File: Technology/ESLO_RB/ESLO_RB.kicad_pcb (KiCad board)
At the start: 4 copper layers, 50.5 x 20 mm, 80 parts, among them CN3 1000pF, CN4 1uF, CN7 1000pF, CN8 1uF, CN9 4700pF, J1 Board to Board, J2 Conn_01x10_Female, U1 TPS62740, U10 MT29F2G01ABBGDWB-IT:G TR, U2 LP5907MFX-1.5, U3 CC2652RB, U4 2450BM14G0011, U5 MAX1720, U6 TPS72301DDCT, U7 ADS1294, U8 LSM303AGR, U9 CY15V104QI-20LPXC

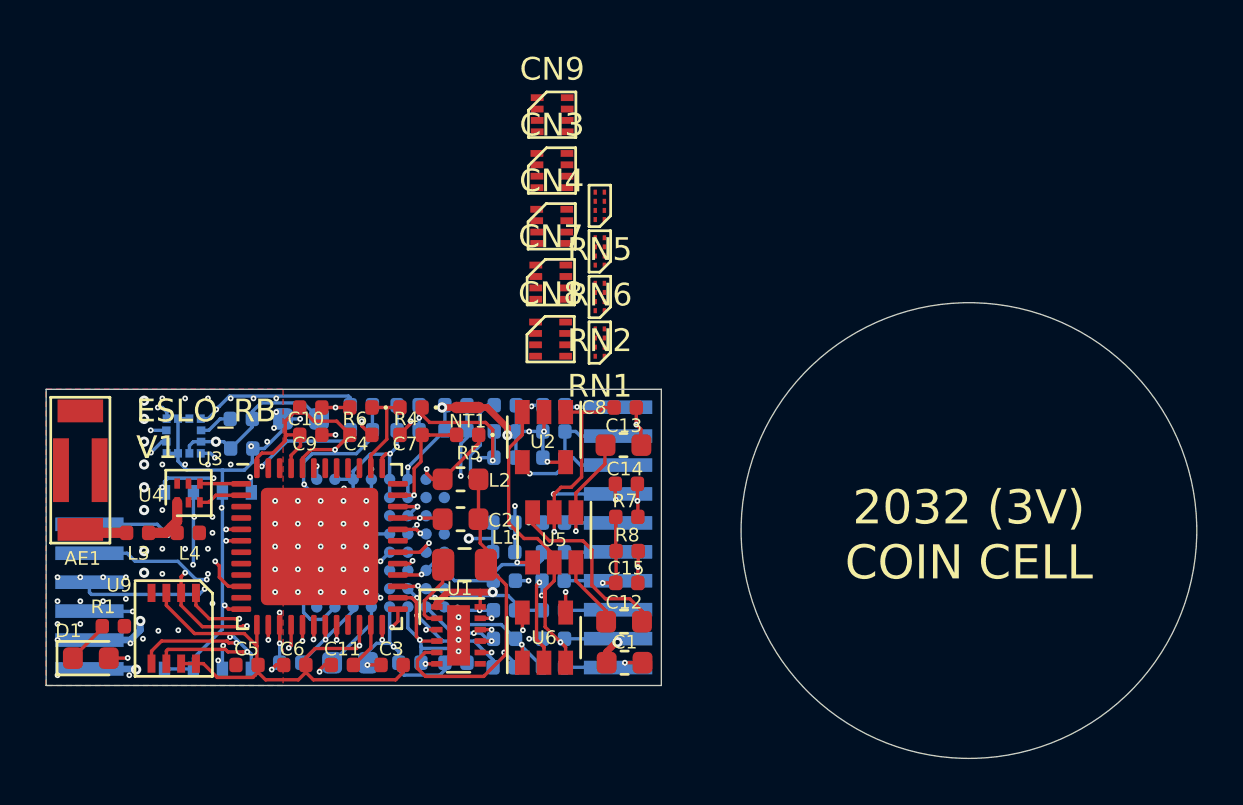
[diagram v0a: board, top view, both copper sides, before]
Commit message: Completed RB design
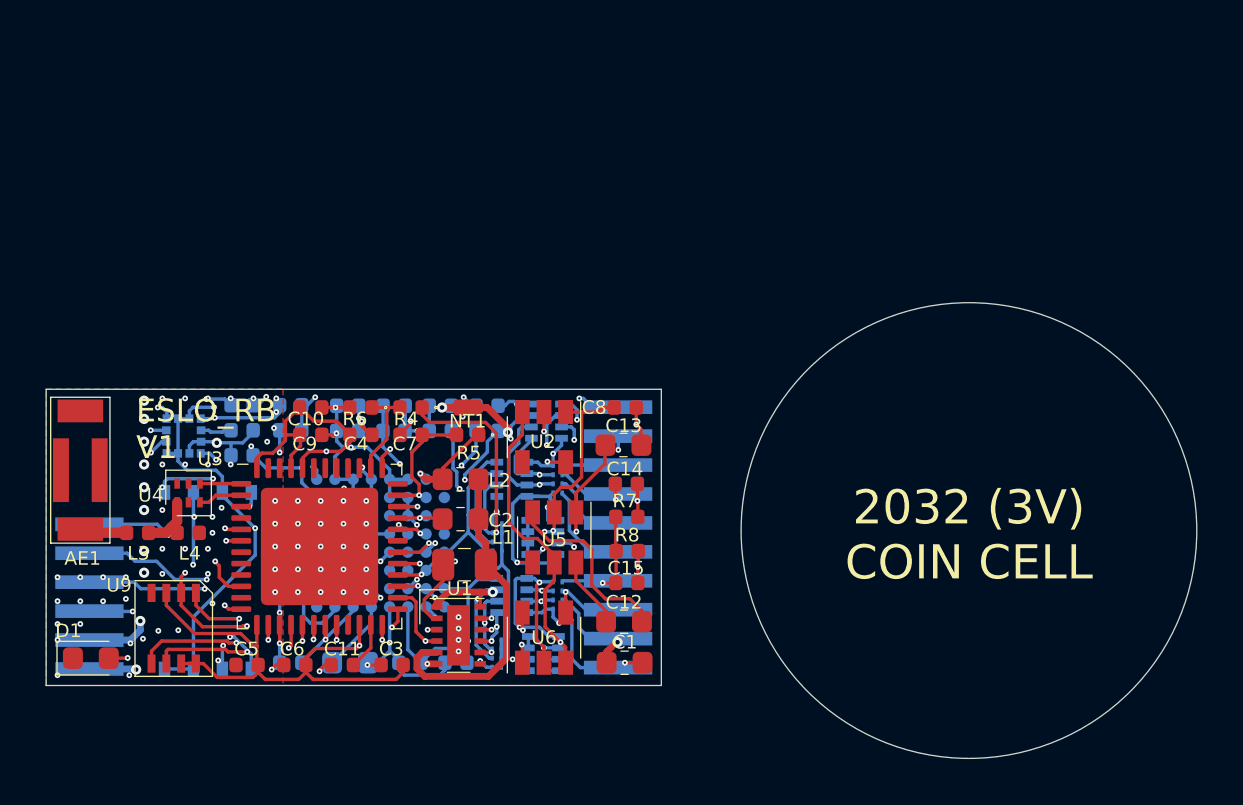
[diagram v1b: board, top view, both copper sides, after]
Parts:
- removed C18, C28: 1uF, Capacitor_SMD:C_0402_1005Metric
- removed C22, C24, C25: 4.7nF, Capacitor_SMD:C_0402_1005Metric
- removed C23: 1000pF, Capacitor_SMD:C_0402_1005Metric
- removed C27: 10uF, Capacitor_SMD:C_0603_1608Metric
- removed R1, R12, R13, R14, R15, R16, R9: 4.7k, Resistor_SMD:R_0402_1005Metric
- removed R10: 1M, Resistor_SMD:R_0402_1005Metric
- CN3, CN4, CN7, CN8, CN9, RN1, RN2, RN5, RN6: moved to B.Cu
- moved RN6 18.2 mm to (144.3, 101.3)
- moved RN5 17.2 mm to (146.9, 98.8), turned to 270 degrees
- moved CN7 16.3 mm to (146.3, 101.3)
- moved CN3 16.1 mm to (146.3, 96.2)
- moved CN9 13.5 mm to (146.5, 91.1), turned to 90 degrees
- moved C19 12.2 mm to (133.1, 92.6)
- moved RN2 11.5 mm to (144.3, 96.2)
- moved CN8 11.4 mm to (144.9, 98.8)
- moved CN4 11.2 mm to (144.9, 93.7)
- moved C35 10.7 mm to (141.8, 91.5), turned to 180 degrees
- moved RN1 6.28 mm to (146.9, 93.7), turned to 270 degrees
- moved C29 5.11 mm to (141.8, 90.4)
- moved C33 5.01 mm to (139.8, 91.5)
- moved C34 5.00 mm to (139.8, 90.4)
- moved R2 3.10 mm to (135.2, 90.4)
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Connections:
- CN3 pad 1: (no net) -> Net-(CN3-Pad1)
- CN3 pad 2: (no net) -> Net-(CN3-Pad2)
- CN3 pad 3: (no net) -> Net-(CN3-Pad3)
- CN3 pad 4: (no net) -> Net-(CN3-Pad4)
- CN3 pad 5: (no net) -> VSSA
- CN3 pad 6: (no net) -> VSSA
- CN3 pad 7: (no net) -> VSSA
- CN3 pad 8: (no net) -> VSSA
- CN4 pad 1: (no net) -> Net-(CN3-Pad1)
- CN4 pad 2: (no net) -> Net-(CN3-Pad2)
- CN4 pad 3: (no net) -> Net-(CN3-Pad3)
- CN4 pad 4: (no net) -> Net-(CN3-Pad4)
- CN4 pad 5: (no net) -> Net-(CN4-Pad5)
- CN4 pad 6: (no net) -> Net-(CN4-Pad6)
- CN4 pad 7: (no net) -> Net-(CN4-Pad7)
- CN4 pad 8: (no net) -> Net-(CN4-Pad8)
- CN7 pad 1: (no net) -> Net-(CN7-Pad1)
- CN7 pad 2: (no net) -> Net-(CN7-Pad2)
- CN7 pad 3: (no net) -> Net-(CN7-Pad3)
- CN7 pad 4: (no net) -> Net-(CN7-Pad4)
- CN7 pad 5: (no net) -> VSSA
- CN7 pad 6: (no net) -> VSSA
- CN7 pad 7: (no net) -> VSSA
- CN7 pad 8: (no net) -> VSSA
- CN8 pad 1: (no net) -> Net-(CN7-Pad1)
- CN8 pad 2: (no net) -> Net-(CN7-Pad2)
- CN8 pad 3: (no net) -> Net-(CN7-Pad3)
- CN8 pad 4: (no net) -> Net-(CN7-Pad4)
- CN8 pad 5: (no net) -> Net-(CN8-Pad5)
- CN8 pad 6: (no net) -> Net-(CN8-Pad6)
- CN8 pad 7: (no net) -> Net-(CN8-Pad7)
- CN8 pad 8: (no net) -> Net-(CN8-Pad8)
- CN9 pad 1: (no net) -> Net-(CN3-Pad2)
- CN9 pad 2: (no net) -> Net-(CN3-Pad3)
- CN9 pad 3: (no net) -> Net-(CN7-Pad1)
- CN9 pad 4: (no net) -> Net-(CN7-Pad3)
- CN9 pad 5: (no net) -> Net-(CN7-Pad4)
- CN9 pad 6: (no net) -> Net-(CN7-Pad2)
- CN9 pad 7: (no net) -> Net-(CN3-Pad4)
- CN9 pad 8: (no net) -> Net-(CN3-Pad1)
- D1 pad 1: Net-(D1-Pad1) -> GNDD
- J2 pad 7: Net-(C23-Pad1) -> Net-(J2-Pad7)
- J2 pad 8: GNDA -> Net-(J2-Pad8)
- R2 pad 1: +1V8 -> VDD
- R3 pad 1: +1V8 -> VDD
- RN1 pad 1: (no net) -> Net-(J2-Pad8)
- RN1 pad 2: (no net) -> Net-(J2-Pad7)
- RN1 pad 3: (no net) -> Net-(J2-Pad6)
- RN1 pad 4: (no net) -> Net-(J2-Pad5)
- RN1 pad 5: (no net) -> Net-(CN3-Pad4)
- RN1 pad 6: (no net) -> Net-(CN3-Pad3)
- RN1 pad 7: (no net) -> Net-(CN3-Pad2)
- RN1 pad 8: (no net) -> Net-(CN3-Pad1)
- RN2 pad 1: (no net) -> Net-(CN4-Pad8)
- RN2 pad 2: (no net) -> Net-(CN4-Pad7)
- RN2 pad 3: (no net) -> Net-(CN4-Pad6)
- RN2 pad 4: (no net) -> Net-(CN4-Pad5)
- RN2 pad 5: (no net) -> Net-(RN2-Pad5)
- RN2 pad 6: (no net) -> Net-(RN2-Pad5)
- RN2 pad 7: (no net) -> Net-(RN2-Pad5)
- RN2 pad 8: (no net) -> Net-(RN2-Pad5)
- RN5 pad 1: (no net) -> Net-(J2-Pad4)
- RN5 pad 2: (no net) -> Net-(J2-Pad3)
- RN5 pad 3: (no net) -> Net-(J2-Pad2)
- RN5 pad 4: (no net) -> Net-(J2-Pad1)
- RN5 pad 5: (no net) -> Net-(CN7-Pad4)
- RN5 pad 6: (no net) -> Net-(CN7-Pad3)
- RN5 pad 7: (no net) -> Net-(CN7-Pad2)
- RN5 pad 8: (no net) -> Net-(CN7-Pad1)
- RN6 pad 1: (no net) -> Net-(CN8-Pad8)
- RN6 pad 2: (no net) -> Net-(CN8-Pad7)
- RN6 pad 3: (no net) -> Net-(CN8-Pad6)
- RN6 pad 4: (no net) -> Net-(CN8-Pad5)
- RN6 pad 5: (no net) -> Net-(RN2-Pad5)
- RN6 pad 6: (no net) -> Net-(RN2-Pad5)
- RN6 pad 7: (no net) -> Net-(RN2-Pad5)
- RN6 pad 8: (no net) -> Net-(RN2-Pad5)
- U7 pad 1E: (no net) -> Net-(CN4-Pad8)
- U7 pad 1F: Net-(C22-Pad1) -> Net-(CN4-Pad6)
- U7 pad 1G: Net-(C24-Pad1) -> Net-(CN8-Pad8)
- U7 pad 1H: Net-(C25-Pad1) -> Net-(CN8-Pad6)
- U7 pad 2E: (no net) -> Net-(CN4-Pad7)
- U7 pad 2F: Net-(C22-Pad2) -> Net-(CN4-Pad5)
- U7 pad 2G: Net-(C24-Pad2) -> Net-(CN8-Pad7)
- U7 pad 2H: Net-(C25-Pad2) -> Net-(CN8-Pad5)
- U7 pad 3A: Net-(C23-Pad1) -> VDDA
- U7 pad 3B: Net-(C23-Pad1) -> Net-(RN2-Pad5)
- U7 pad 3C: Net-(C23-Pad2) -> Net-(RN2-Pad5)
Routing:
- net Net-(CN7-Pad4): track 0.00 -> 16.2 mm, vias 0 -> 3
- net Net-(CN7-Pad2): track 0.00 -> 15.8 mm, vias 0 -> 3
- net Net-(CN7-Pad1): track 0.00 -> 15.8 mm, vias 0 -> 2
- net Net-(CN7-Pad3): track 0.00 -> 14.6 mm, vias 0 -> 3
- net Net-(C23-Pad1): track 14.4 -> 0.00 mm, vias 2 -> 0
- net Net-(RN2-Pad5): track 0.00 -> 13.6 mm, vias 0 -> 2
- net Net-(CN3-Pad4): track 0.00 -> 12.1 mm, vias 0 -> 2
- net VSSA: track 22.1 -> 32.9 mm, vias 10 -> 14
- net Net-(C22-Pad2): track 9.81 -> 0.00 mm, vias 3 -> 0
- net Net-(CN3-Pad3): track 0.00 -> 9.12 mm, vias 0 -> 2
- net Net-(CN3-Pad2): track 0.00 -> 7.16 mm, vias 0 -> 2
- net Net-(CN4-Pad7): track 0.00 -> 7.02 mm, vias 0 -> 2
- net Net-(C24-Pad2): track 7.00 -> 0.00 mm, vias 4 -> 0
- net Net-(C25-Pad2): track 6.75 -> 0.00 mm, vias 2 -> 0
- net Net-(CN4-Pad8): track 0.00 -> 6.68 mm
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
